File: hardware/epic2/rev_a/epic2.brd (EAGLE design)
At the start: 22.1 x 14.6 mm, 34 parts, among them U1 RV-4162-C7, U2 FM25LBTDFN-8, U3 CC2538, X1 EPSON-FA-128, X3 ABS05-32.768KHZ-T

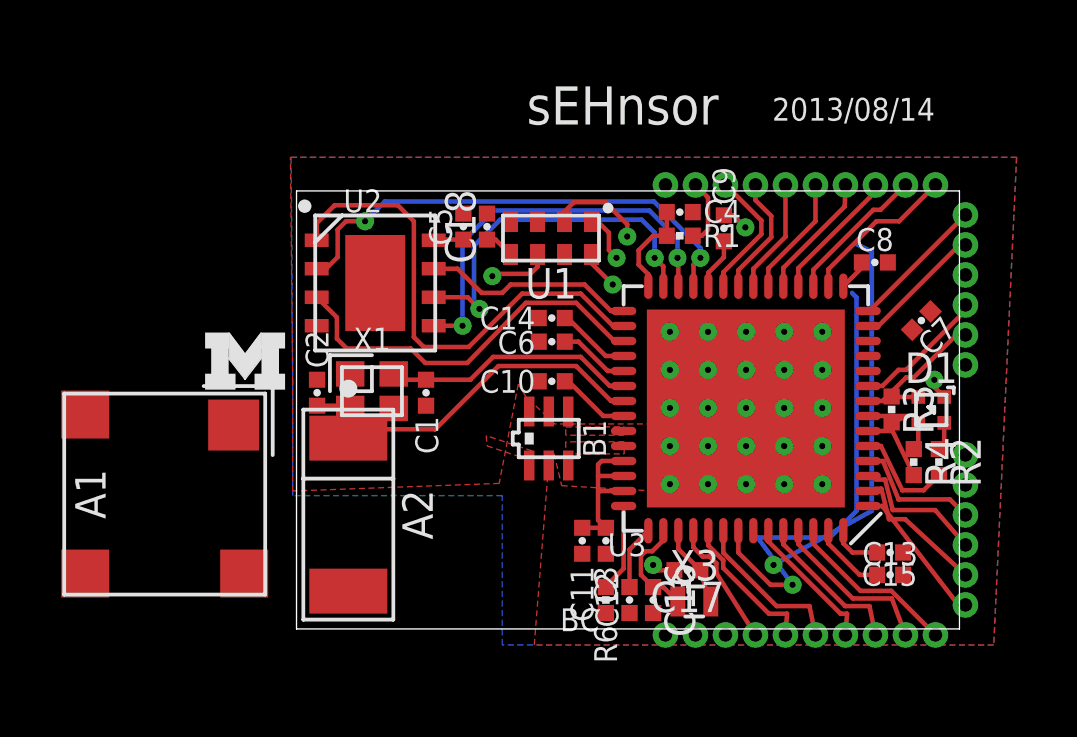
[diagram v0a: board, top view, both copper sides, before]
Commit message: workin on epic2
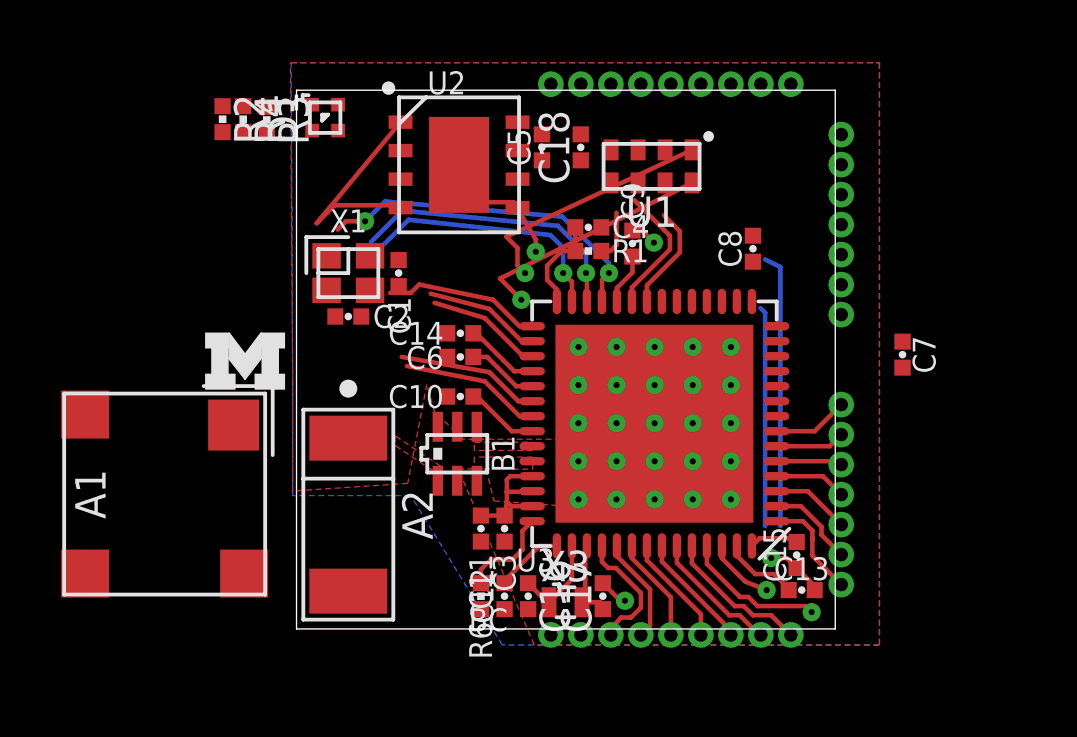
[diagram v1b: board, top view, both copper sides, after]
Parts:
- removed U$2: EPIC2-HEADER, epic2:EPIC2-HEADER
- added J1: EPIC2-HEADER2, epic2:EPIC2-HEADER2
- moved R2 26.5 mm to (-2.46, 17.0)
- moved R4 25.1 mm to (-1.78, 17.0)
- moved R3 23.0 mm to (-0.99, 17.0)
- moved D1 22.4 mm to (0.95, 17.0), turned to 90 degrees
- moved U2 4.83 mm to (5.42, 15.5)
- moved X3 4.29 mm to (8.97, 0.89)
- moved C12 4.17 mm to (6.93, 1.09)
- moved C16 4.17 mm to (7.72, 1.09)
- moved R6 4.17 mm to (6.15, 1.09)
- moved U1 4.12 mm to (11.8, 15.4)
- moved C18 4.09 mm to (9.47, 16.1)
- moved C1 4.09 mm to (3.40, 11.9)
- moved C8 4.09 mm to (15.2, 12.7), turned to 90 degrees
- moved X1 4.01 mm to (1.73, 11.9)
- moved C5 3.72 mm to (8.18, 16.1)
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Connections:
- removed net B1: U$2.10, U3.54
- removed net B2: U$2.9, U3.53
- removed net UNUSED2: U$2.3
- new net B5: J1.7, U3.50
- new net B6: J1.6, U3.49
- net !RESET: now also J1.31; no longer U$2.31
- net !RTC_INT: now also U3.54; no longer U3.49
- net ADC3: now also J1.26; no longer U$2.26
- net ADC4: now also J1.27; no longer U$2.27
- net ADC5: now also J1.28; no longer U$2.28
- net ADC6: now also J1.29; no longer U$2.29
- net ADC7: now also J1.30; no longer U$2.30
- net B3: now also J1.9; no longer U$2.8
- net B4: now also J1.8; no longer U$2.7
- net BOOTLOADER_CTRL: now also J1.25; no longer U$2.25
- net BOOTLOADER_RX: now also J1.23; no longer U$2.23
- net BOOTLOADER_TX: now also J1.24; no longer U$2.24
- net C0: now also J1.22; no longer U$2.22
- net C1: now also J1.21; no longer U$2.21
- net C2: now also J1.20; no longer U$2.20
- net C3: now also J1.19
- net DGND_USB: now also J1.10; no longer U$2.11
- net DVDD_USB: now also J1.13; no longer U$2.14
- net GND: now also J1.32; no longer U$2.32
- net I2C_SCL: now also J1.17; no longer U$2.18
- net I2C_SDA: now also J1.18; no longer U$2.19
- net LED_BLUE: no longer U3.6
- net LED_GREEN: no longer U3.7
- net LED_RED: no longer U3.5
- net RTC_CLKOUT: now also U3.53; no longer U3.50
- net SPI_MISO: now also J1.14, U3.5; no longer U$2.15
- net SPI_MOSI: now also J1.15, U3.6; no longer U$2.16
- net SPI_SCK: now also J1.16, U3.7; no longer U$2.17
- net TCK: now also J1.4; no longer U$2.5
- net TDO: now also J1.5; no longer U$2.6
- net TMS: now also J1.3; no longer U$2.4
- net UNUSED1: now also J1.2; no longer U$2.2
- net USB_N: now also J1.12; no longer U$2.13
- net USB_P: now also J1.11; no longer U$2.12
- net VCC: now also J1.1; no longer U$2.1
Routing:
- net !FRAM_WP: track 12.9 -> 3.86 mm
- net !RTC_INT: track 18.4 -> 9.61 mm, vias 2 -> 1
- net N$10: track 11.9 -> 4.70 mm
- net B1: track 5.76 -> 0.00 mm
- net B2: track 5.61 -> 0.00 mm
- net BOOTLOADER_RX: track 5.30 -> 0.00 mm
- net !FRAM_CS: track 16.4 -> 11.2 mm
- net BOOTLOADER_TX: track 4.79 -> 0.00 mm
- net C0: track 4.57 -> 0.04 mm
- net VCC: track 20.5 -> 16.0 mm, vias 1 -> 0
- net BOOTLOADER_CTRL: track 4.45 -> 0.00 mm
- net ADC3: track 4.22 -> 0.00 mm
- net ADC4: track 4.03 -> 0.00 mm
- net C1: track 4.36 -> 0.34 mm
- net B5: track 0.00 -> 3.92 mm
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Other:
- board size 22.1 x 14.6 mm -> 18 x 18 mm
- board text removed: "2013/08/14"
- board text removed: "sEHnsor"
